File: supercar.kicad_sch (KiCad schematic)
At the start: 59 parts, among them U1 74HC283, U2 74HC574, U3 74HC154, U4 74HC574, U5 74HC21, U6 74HC02, U7 74HC04, U8 NE555D

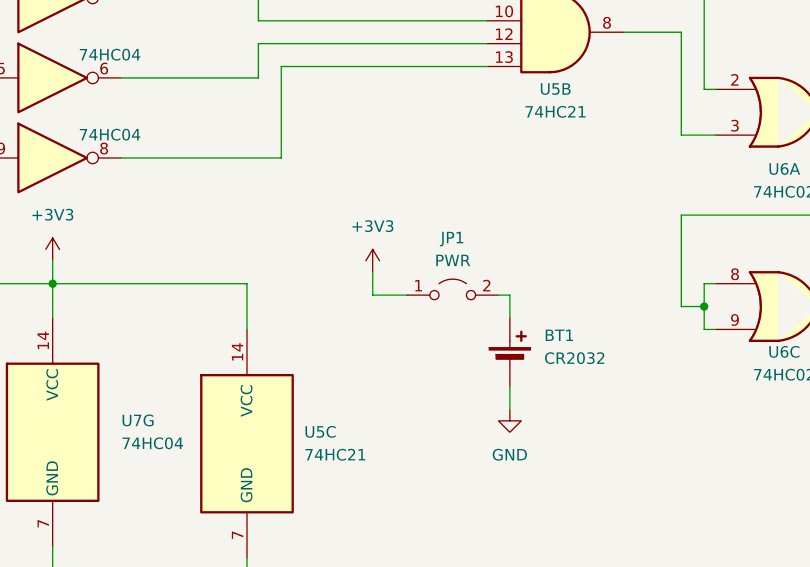
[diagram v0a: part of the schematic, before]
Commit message: Update schematic and PCB
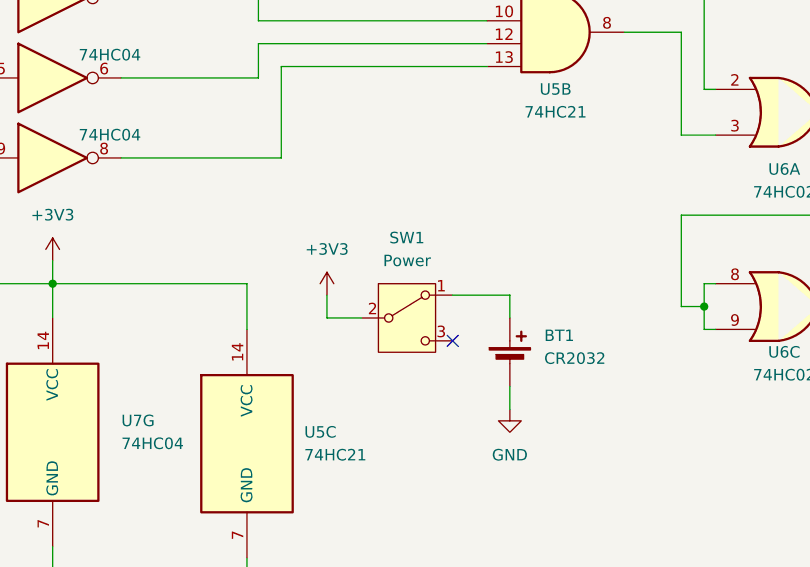
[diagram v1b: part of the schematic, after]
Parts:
- removed JP1: PWR, Connector_PinHeader_2.54mm:PinHeader_1x02_P2.54mm_Vertical, symbol Jumper:Jumper_2_Open
- added SW1: Power, Button_Switch_THT:SW_Slide_1P2T_CK_OS102011MS2Q, symbol Switch:SW_SPDT
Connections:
- net +3V3: now also SW1.2 (B)
- net at BT1.1 (+): now also SW1.1 (A)
- no-connect marks 11 -> 12
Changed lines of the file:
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@@
   (no_connect (at 187.96 52.07))
   (no_connect (at 189.23 128.27))
+  (no_connect (at 95.25 163.83))
   (no_connect (at 137.16 52.07))
   (no_connect (at 80.01 25.4))
@@
     (stroke (width 0) (type default))
   )
-  (wire (pts (xy 90.17 158.75) (xy 86.36 158.75))
+  (wire (pts (xy 85.09 161.29) (xy 81.28 161.29))
     (stroke (width 0) (type default))
   )
@@
     (stroke (width 0) (type default))
   )
-  (wire (pts (xy 100.33 158.75) (xy 101.6 158.75))
-    (stroke (width 0) (type default))
-  )
   (wire (pts (xy 214.63 107.95) (xy 214.63 110.49))
     (stroke (width 0) (type default))
@@
     (stroke (width 0) (type default))
   )
+  (wire (pts (xy 95.25 158.75) (xy 101.6 158.75))
+    (stroke (width 0) (type default))
+  )
   (wire (pts (xy 86.36 44.45) (xy 86.36 121.92))
     (stroke (width 0) (type default))
@@
     (stroke (width 0) (type default))
   )
-  (wire (pts (xy 86.36 156.21) (xy 86.36 158.75))
+  (wire (pts (xy 81.28 158.75) (xy 81.28 161.29))
     (stroke (width 0) (type default))
   )
@@
     )
   )
-  (symbol (lib_id "Jumper:Jumper_2_Open") (at 95.25 158.75 0) (unit 1)
-    (in_bom yes) (on_board yes) (dnp no) (fields_autoplaced)
-    (property "Reference" "JP1" (at 95.25 152.4 0)
-      (effects (font (size 1.27 1.27)))
-    )
-    (property "Value" "PWR" (at 95.25 154.94 0)
-      (effects (font (size 1.27 1.27)))
-    )
-    (property "Footprint" "Connector_PinHeader_2.54mm:PinHeader_1x02_P2.54mm_Vertical" (at 95.25 158.75 0)
-      (effects (font (size 1.27 1.27)) hide)
-    )
-    (property "Datasheet" "~" (at 95.25 158.75 0)
-      (effects (font (size 1.27 1.27)) hide)
-    )
-    (pin "2")
-    (pin "1")
-    (instances
-      (project "supercar"
-        (path "/6cdc46ee-6809-405f-bf74-06040b593f5f"
-          (reference "JP1") (unit 1)
-        )
-      )
-    )
-  )
   (symbol (lib_id "Device:R_Small") (at 255.27 62.23 90) (mirror x) (unit 1)
     (in_bom yes) (on_board yes) (dnp no)
@@
     )
   )
-  (symbol (lib_id "power:+3V3") (at 86.36 156.21 0) (unit 1)
+  (symbol (lib_id "power:+3V3") (at 81.28 158.75 0) (unit 1)
     (in_bom yes) (on_board yes) (dnp no) (fields_autoplaced)
-    (property "Reference" "#PWR020" (at 86.36 160.02 0)
+    (property "Reference" "#PWR020" (at 81.28 162.56 0)
       (effects (font (size 1.27 1.27)) hide)
     )
-    (property "Value" "+3V3" (at 86.36 151.13 0)
+    (property "Value" "+3V3" (at 81.28 153.67 0)
       (effects (font (size 1.27 1.27)))
     )
-    (property "Footprint" "" (at 86.36 156.21 0)
+    (property "Footprint" "" (at 81.28 158.75 0)
       (effects (font (size 1.27 1.27)) hide)
     )
-    (property "Datasheet" "" (at 86.36 156.21 0)
+    (property "Datasheet" "" (at 81.28 158.75 0)
       (effects (font (size 1.27 1.27)) hide)
     )
@@
         )
       )
+    )
+  )
+  (symbol (lib_id "Switch:SW_SPDT") (at 90.17 161.29 0) (unit 1)
+    (in_bom yes) (on_board yes) (dnp no) (fields_autoplaced)
+    (property "Reference" "SW1" (at 90.17 152.4 0)
+      (effects (font (size 1.27 1.27)))
+    )
+    (property "Value" "Power" (at 90.17 154.94 0)
+      (effects (font (size 1.27 1.27)))
+    )
+    (property "Footprint" "Button_Switch_THT:SW_Slide_1P2T_CK_OS102011MS2Q" (at 90.17 161.29 0)
+      (effects (font (size 1.27 1.27)) hide)
+    )
+    (property "Datasheet" "~" (at 90.17 168.91 0)
+      (effects (font (size 1.27 1.27)) hide)
+    )
+    (pin "2")
+    (pin "1")
+    (pin "3")
+    (instances
+      (project "supercar"
+        (path "/6cdc46ee-6809-405f-bf74-06040b593f5f"
+          (reference "SW1") (unit 1)
+        )
+      )
